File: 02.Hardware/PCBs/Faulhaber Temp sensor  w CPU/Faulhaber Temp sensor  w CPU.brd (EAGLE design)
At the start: 21.9 x 23.2 mm, 16 parts, among them IC1 MCP9700T-E_TT, IC2 ATTINY85V-10SUR, Q2 SI2393DS-T1-GE3, Q3 2N7002PW, U7 AP2205-33W5-7

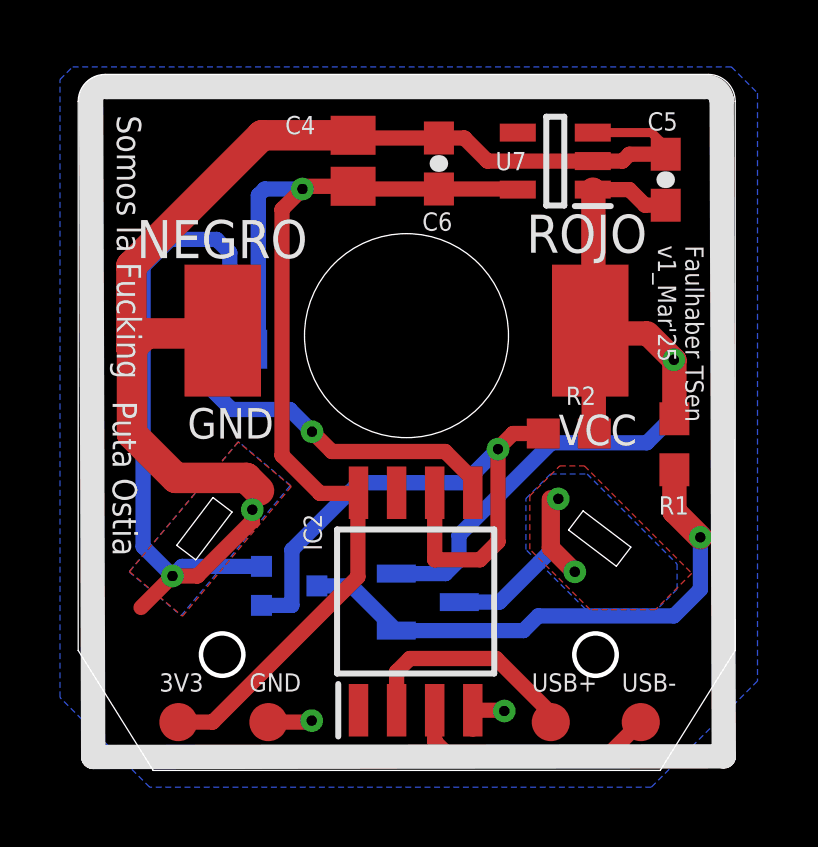
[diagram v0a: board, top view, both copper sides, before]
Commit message: Sensado de voltaje de entrada. version 2
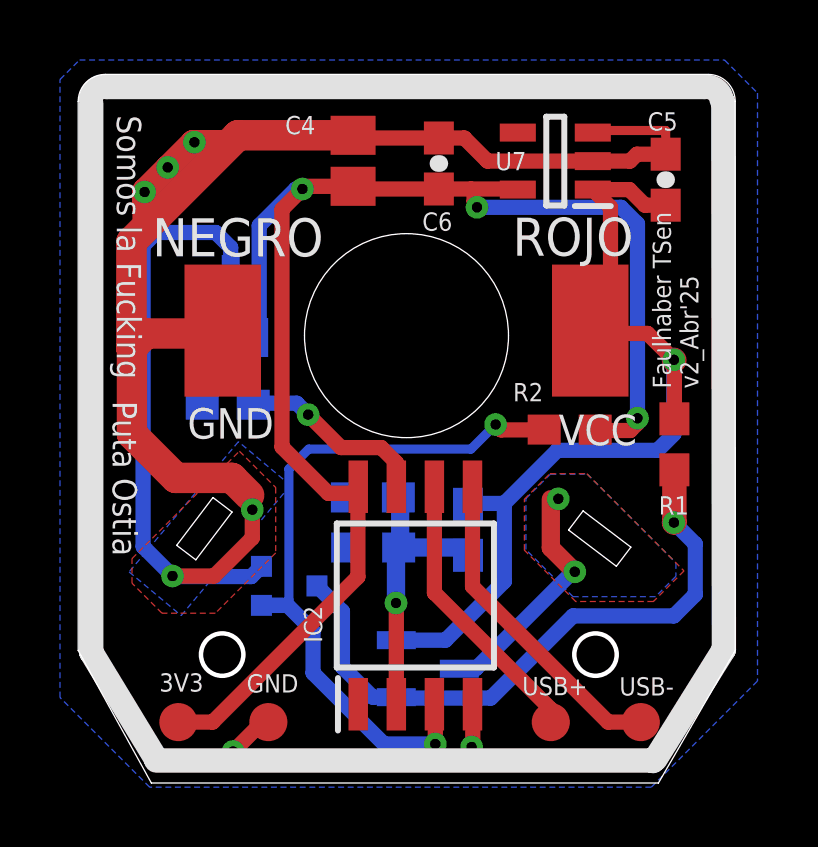
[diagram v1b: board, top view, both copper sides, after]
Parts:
- added C8: 100n, SparkFun-Capacitors:0603
- added R3: (no value), SparkFun-Resistors:0603
- added R4: 169k, SparkFun-Resistors:0603
- added R5: 39k, SparkFun-Resistors:0603
- R1: value 100K -> (none)
- R2: value 33K -> (none)
- moved Q2 2.22 mm to (108.2, 73.1)
- moved IC1 0.39 mm to (101.6, 85.2)
- moved IC2 0.20 mm to (107.8, 75.5)
- moved R2 0.13 mm to (112.9, 81.0)
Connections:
- new net N$1: IC1.2, R3.1
- new net VOUTSENSE: C8.1, IC2.2, R4.2, R5.1
- net 3V3: now also R2.2
- net GND: now also C8.2, R5.2
- net ROJO: now also R4.1; no longer R2.2
- net SW_OUT: now also IC2.3; no longer IC2.6
- net USB+: now also IC2.6; no longer IC2.2
- net USB-: now also IC2.5; no longer IC2.3
- net VTEMP: now also IC2.7, R3.2; no longer IC1.2, IC2.5
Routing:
- net 3V3: track 37.0 -> 50.7 mm, vias 1 -> 3
- net VOUTSENSE: track 0.00 -> 9.54 mm, vias 0 -> 1
- net GND: track 63.7 -> 70.1 mm, vias 4 -> 7
- net VTEMP: track 11.9 -> 6.42 mm
- net SW_OUT: track 20.5 -> 24.4 mm, vias 1 -> 2
- net N$3: track 18.3 -> 21.1 mm
- net USB-: track 8.50 -> 10.8 mm
- net N$1: track 0.00 -> 2.24 mm
- net USB+: track 7.66 -> 9.45 mm
- net ROJO: track 29.7 -> 30.3 mm
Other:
- board size 21.9 x 23.2 mm -> 21.9 x 23.6 mm
- board text added: "Faulhaber TSen v2_Abr'25"
- board text removed: "Faulhaber TSen v1_Mar'25"
